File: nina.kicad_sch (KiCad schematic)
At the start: 10 parts, among them P5 GRPB042VWVN-RC

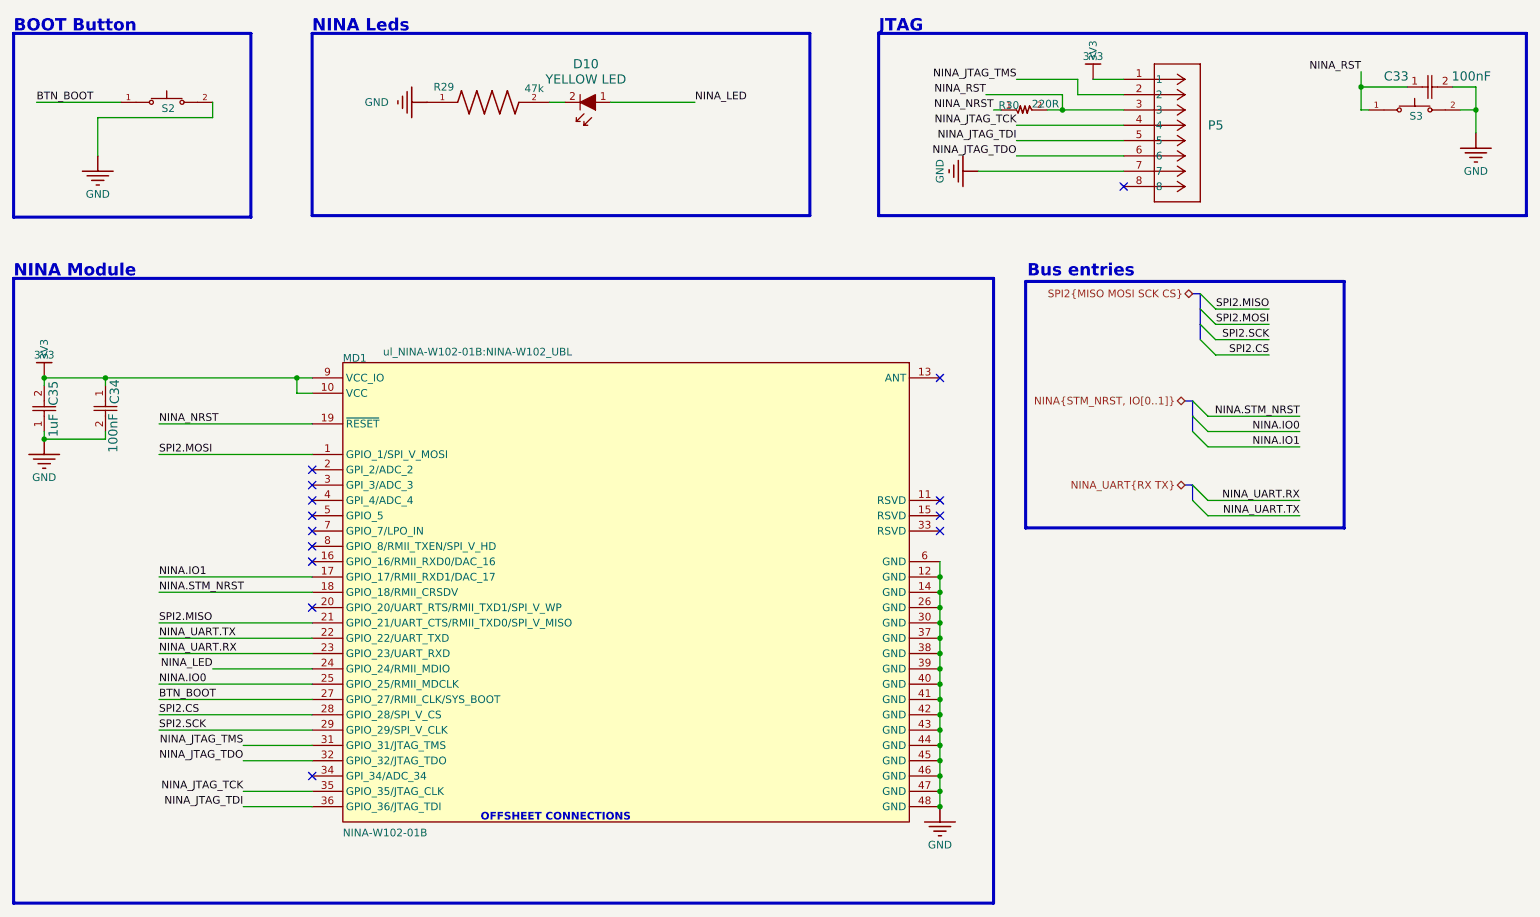
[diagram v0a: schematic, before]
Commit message: power planes
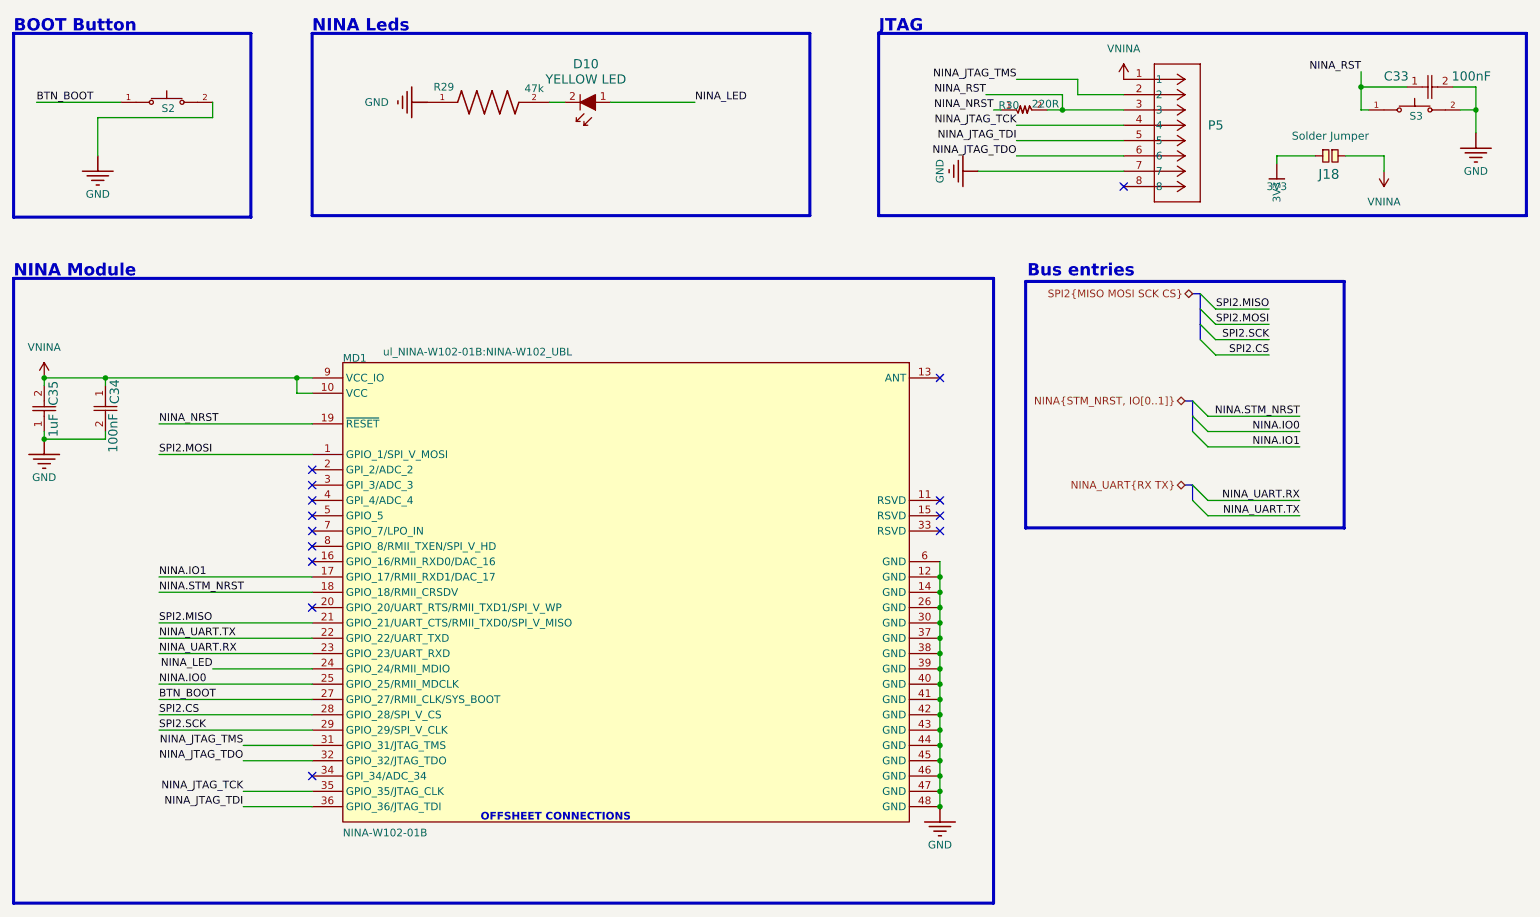
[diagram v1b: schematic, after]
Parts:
- added J18: Solder Jumper, Jumper:SolderJumper-2_P1.3mm_Open_RoundedPad1.0x1.5mm, symbol gap9_deck:CMP-00005-5
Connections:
- net 3V3: now also J18.2; no longer C34.1, C35.2, MD1.10 (VCC), MD1.9 (VCC_IO), P5.1
- new net VNINA: C34.1, C35.2, J18.1, MD1.10 (VCC), MD1.9 (VCC_IO), P5.1
